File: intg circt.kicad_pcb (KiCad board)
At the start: 4 copper layers, 18.2 x 40.8 mm, 55 parts, among them J1 Conn_01x01_Pin, J2 USB_C_Receptacle_USB2.0_16P, J3 Conn_01x02_Pin, J4 5033981892, J5 Conn_01x02_Pin, J6 Conn_01x01_Pin, U1 ESP32-S3-MINI-1U, U2 MAXM86161EFD_T, U3 BMI270, U4 BQ24074RGT, U6 USBLC6-2P6, U7 MAX17048X+T10, U8 TLV75533PDBV, U9 LMV358IDR

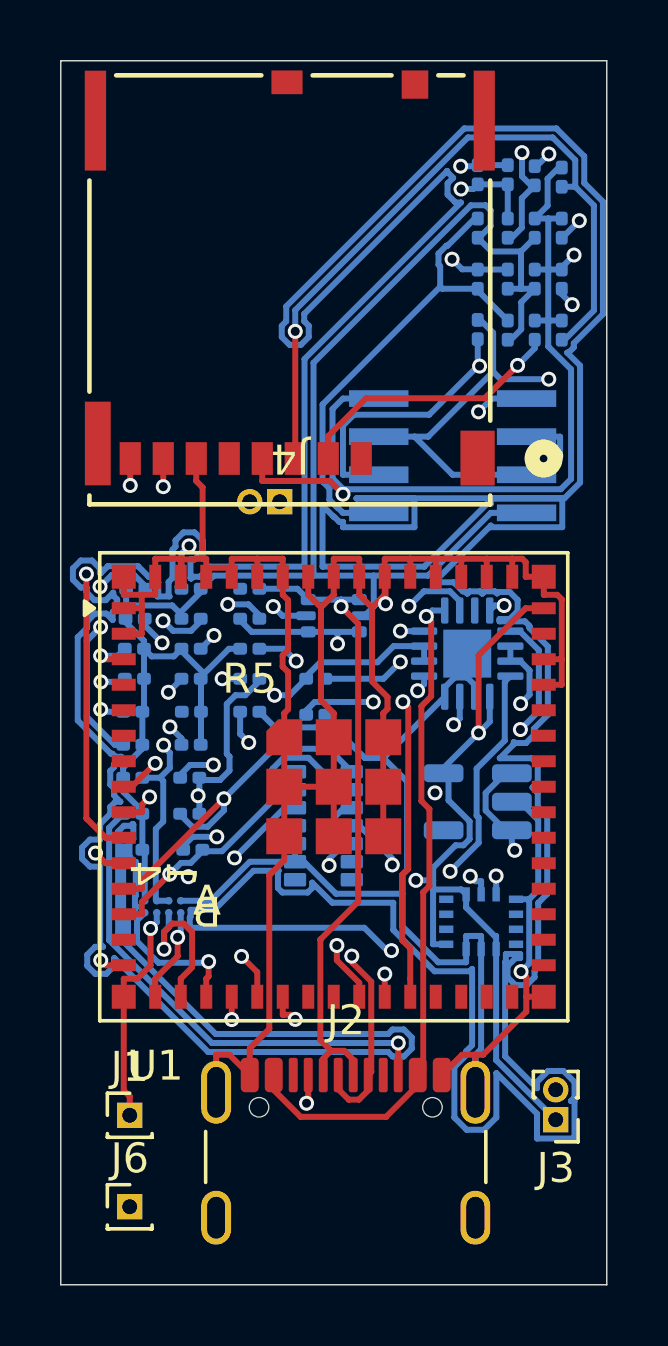
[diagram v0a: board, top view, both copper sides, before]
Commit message: placement and routing
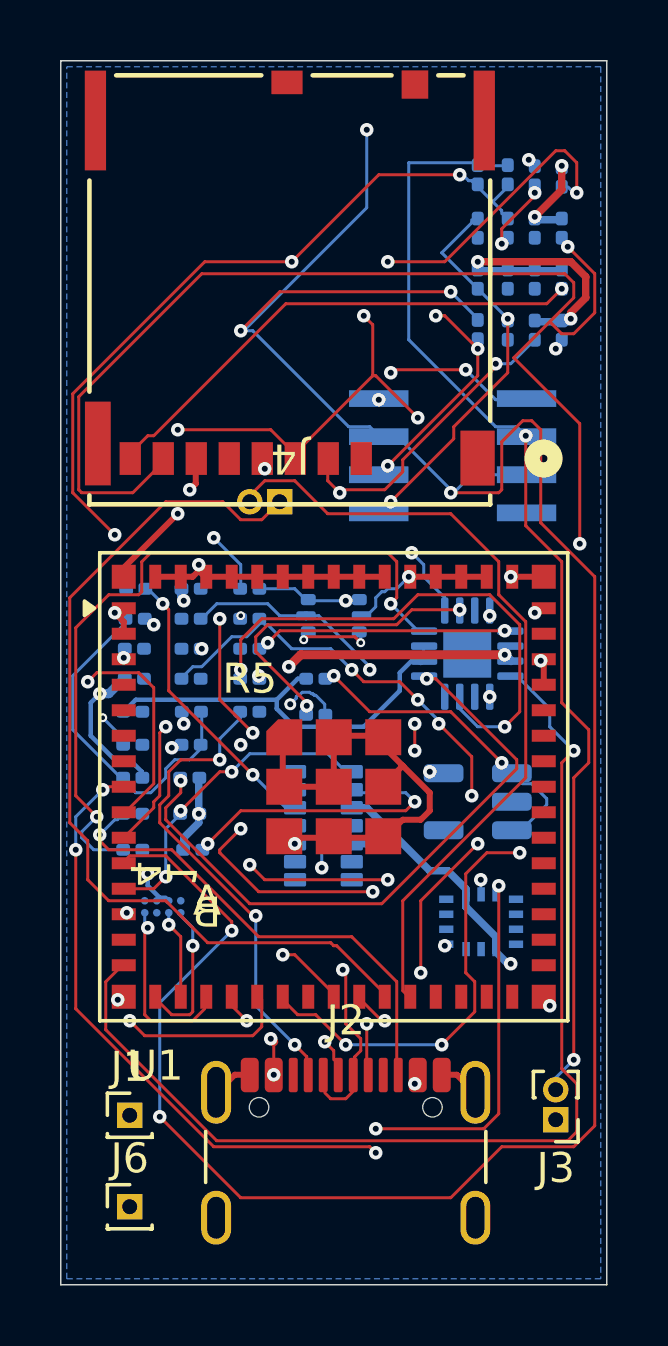
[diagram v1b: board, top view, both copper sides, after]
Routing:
- net Net-(U4-ILIM): track 233.5 -> 24.5 mm
- net GND: track 214.0 -> 58.7 mm, vias 3 -> 11
- net +3V3: track 131.7 -> 32.7 mm, vias 11 -> 16
- net /OUT_B: track 49.1 -> 93.1 mm, vias 3 -> 7
- net /J1_DAT0: track 42.5 -> 65.7 mm, vias 3 -> 5
- net /USB_D-: track 0.00 -> 20.7 mm, vias 0 -> 3
- net /U3_SDX: track 14.9 -> 33.5 mm, vias 2 -> 5
- net /~{CE}: track 21.6 -> 36.4 mm, vias 2 -> 1
- net /VREF: track 23.2 -> 9.61 mm
- net /Temp_SDA: track 17.9 -> 30.0 mm, vias 1 -> 0
- net /U3_SCX: track 14.0 -> 24.7 mm, vias 2 -> 4
- net /~{PGOOD}: track 28.0 -> 17.4 mm
- net /J1_CD: track 40.9 -> 32.1 mm, vias 2 -> 3
- net /OUT_A: track 37.2 -> 45.5 mm, vias 3 -> 6
- net /VBUS: track 50.5 -> 42.6 mm, vias 4 -> 7
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- added copper zone on In2.Cu, net +3V3
- added copper zone on B.Cu, net GND
- added copper zone on In1.Cu, net GND
